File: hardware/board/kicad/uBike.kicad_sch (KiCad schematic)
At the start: 22 parts, among them J2 F31S-1A7L1-11040, Q1 MMBT3904, U3 MDBT50Q-P1MV2, X1 32.768kHz

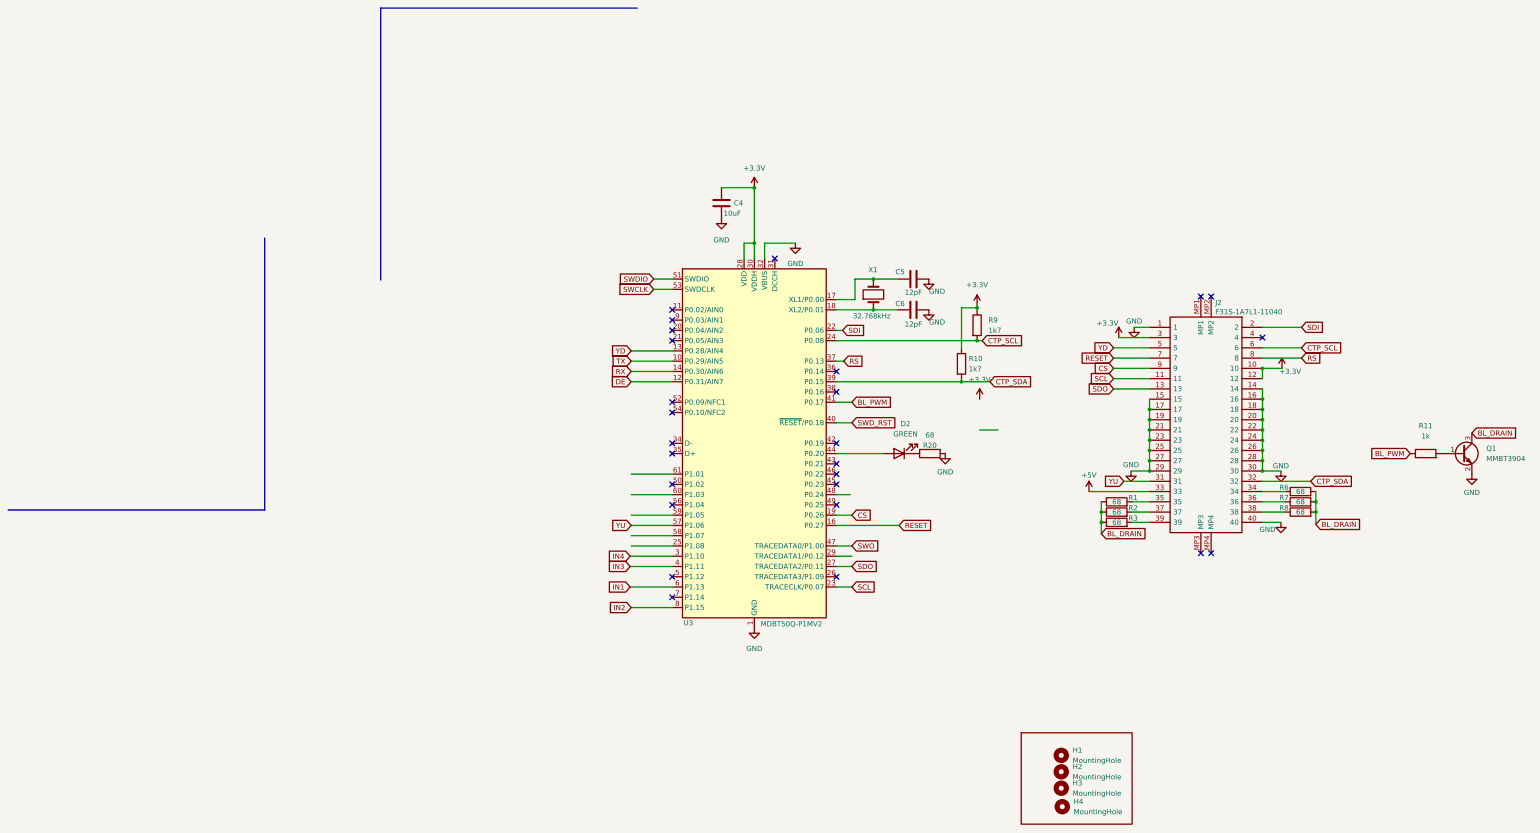
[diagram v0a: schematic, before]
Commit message: Schematic cleanup
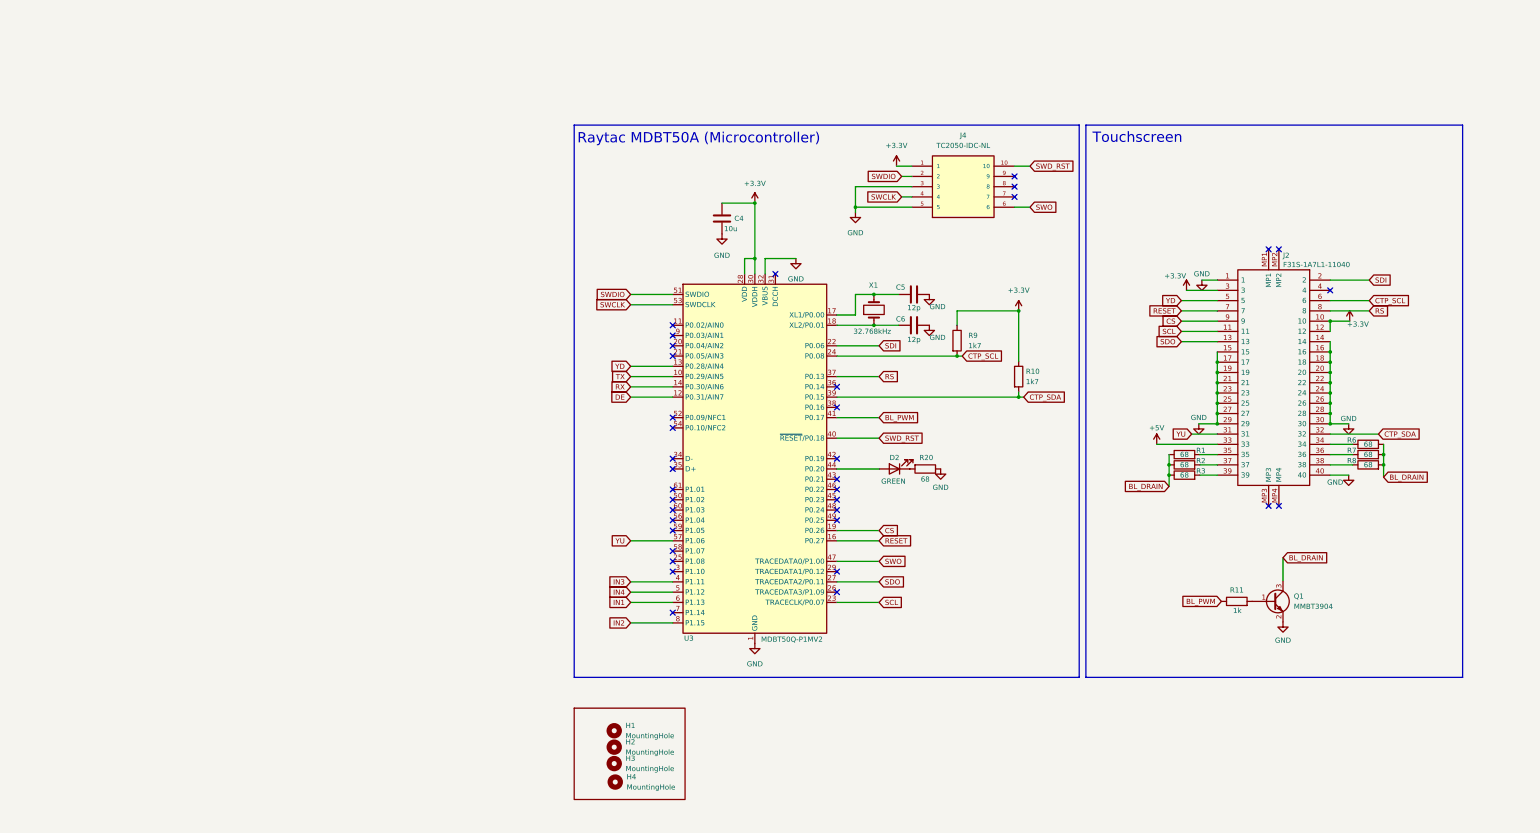
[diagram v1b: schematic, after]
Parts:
- added J4: TC2050-IDC-NL, Connector:Tag-Connect_TC2050-IDC-NL_2x05_P1.27mm_Vertical, symbol TC2050-IDC-NL:TC2050-IDC-NL
- C4: value 10uF -> 10u
- C5, C6: value 12pF -> 12p
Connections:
- net +3.3V: now also J4.1
- net GND: now also J4.3, J4.5
- net IN4: now also U3.5 (P1.12); no longer U3.3 (P1.10)
- net SWCLK: now also J4.4
- net SWDIO: now also J4.2
- net SWD_RST: now also J4.10
- net SWO: now also J4.6
- no-connect marks 26 -> 36
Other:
- note added: "Raytac MDBT50A (Microcontroller)"
- note added: "Touchscreen"
- moved on the sheet: C4, C5, C6, D2, H1, H2, H3, H4, J2, Q1, R1, R10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
